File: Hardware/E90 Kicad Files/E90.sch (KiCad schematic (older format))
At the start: 108 parts, among them J1 Conn_01x03, J10 SJ-63073E, J2 SWD Connector Conn_02x03, J3 Power Test Point Conn_01x02, J4 Conn_01x03, J5 Conn_01x02, J6 Conn_01x03, J7 USB_B_Mini, J8 Barrel_Jack_Switch, J9 SJ-63073E, U1 AMS1117-3.3, U2 CS4344_CZZ, U3 TLV2774, U4 CS5343_CZZ, U5 STM32F407VGT60, U6 USBLC6-2SC6

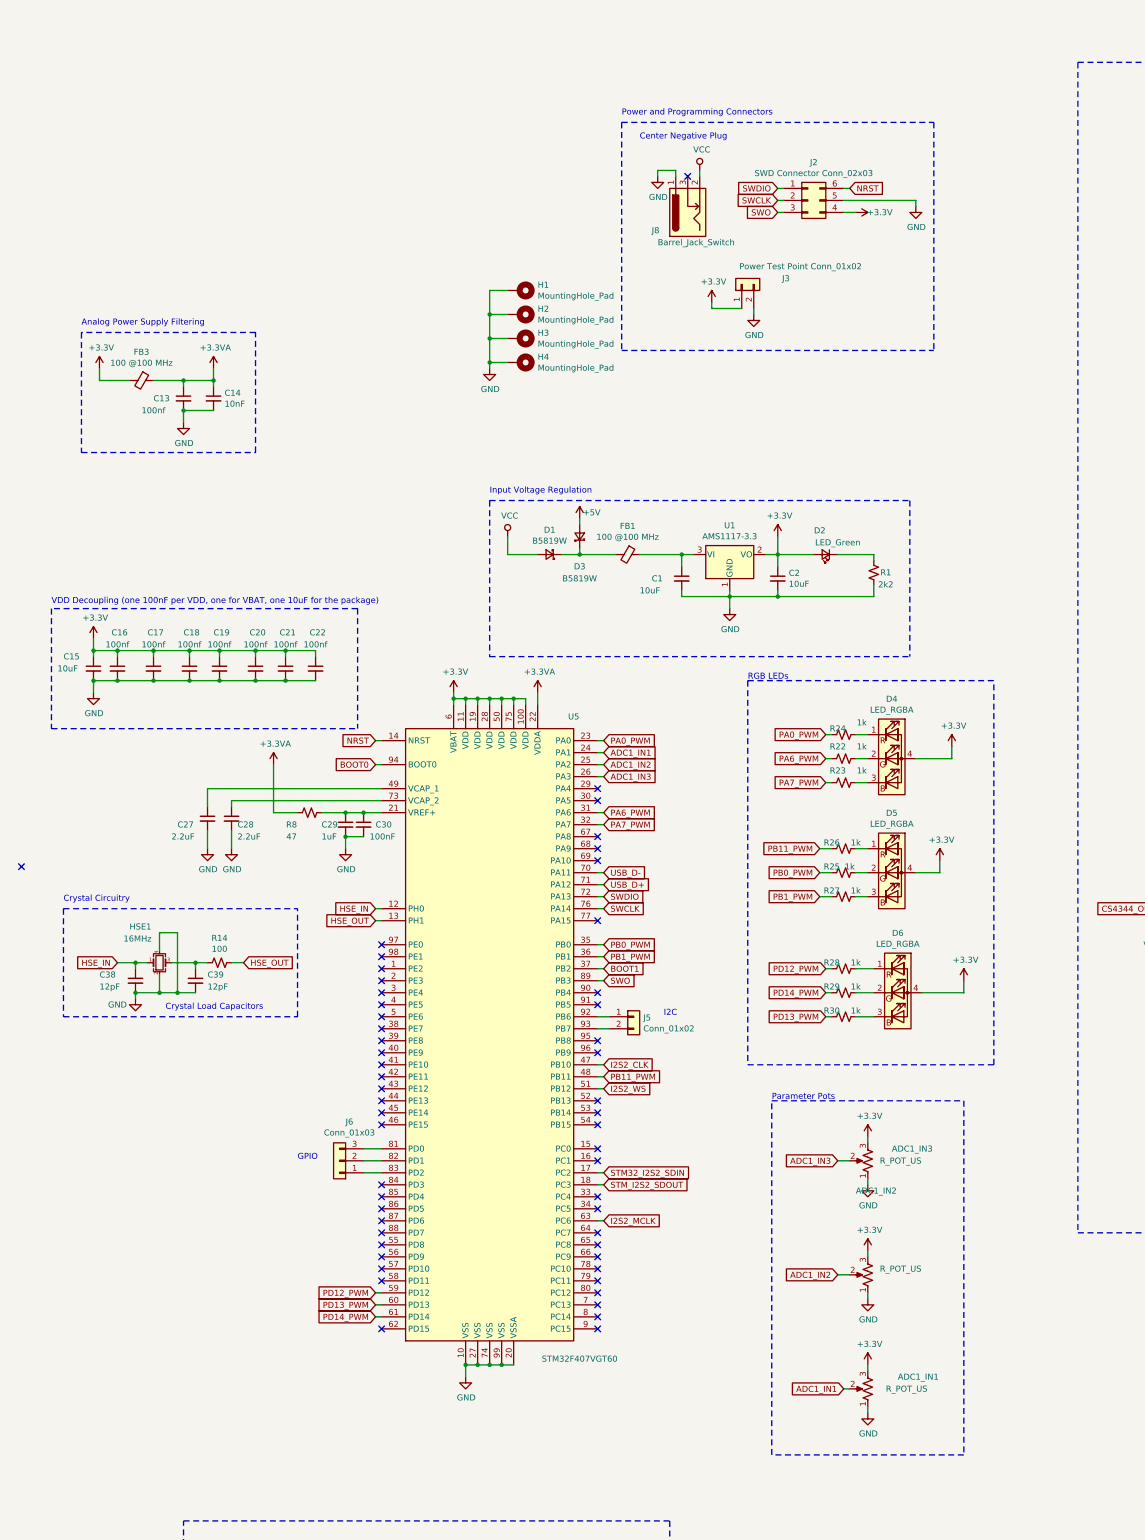
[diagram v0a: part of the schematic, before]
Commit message: iir
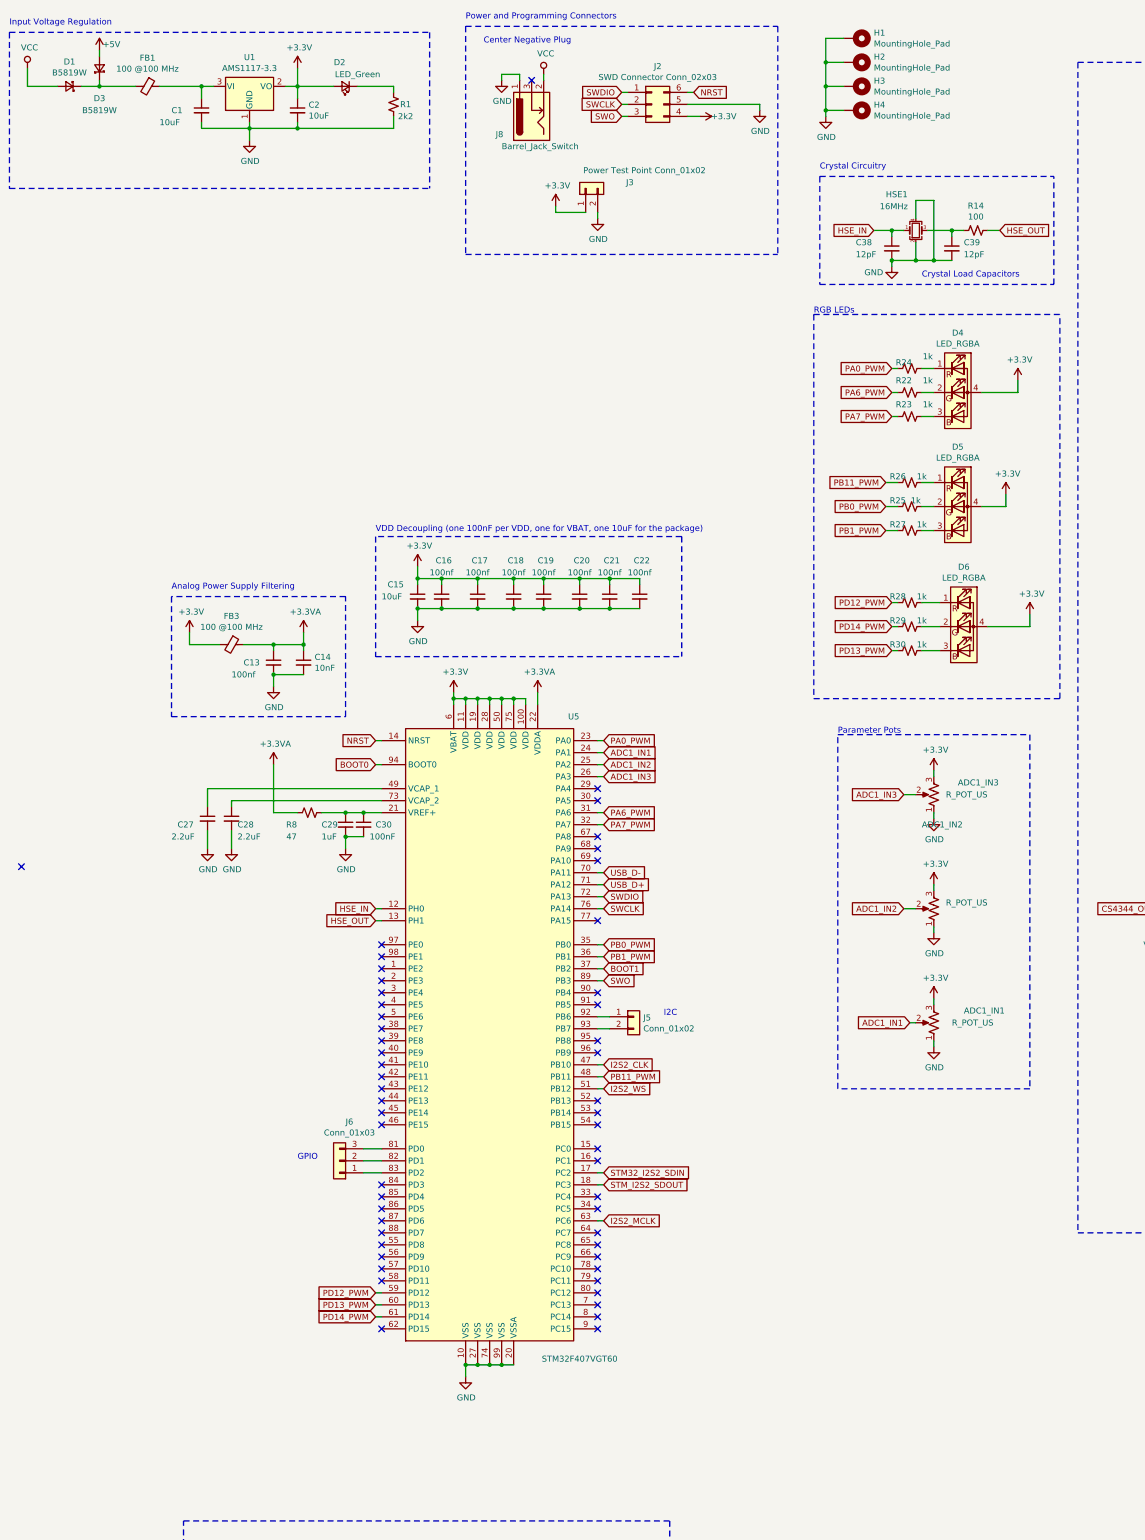
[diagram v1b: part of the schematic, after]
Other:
- moved on the sheet: ADC1_IN1, ADC1_IN2, ADC1_IN3, C1, C13, C14, C15, C16, C17, C18, C19, C2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
